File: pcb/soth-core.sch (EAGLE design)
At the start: 1 part, among them U1 ATXMEGA32D4-AU

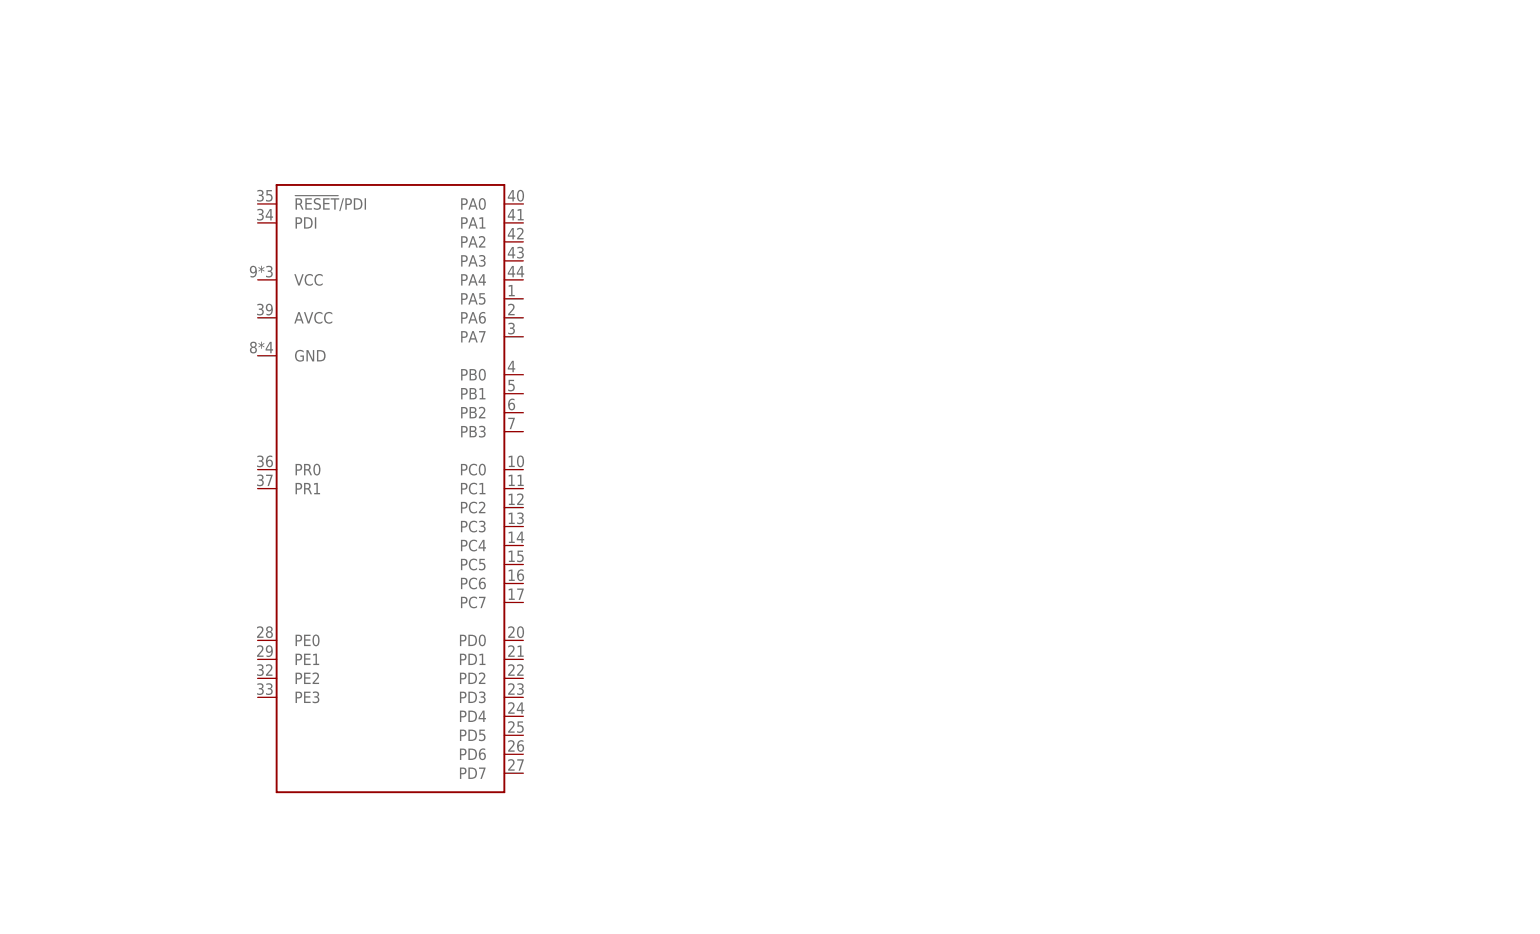
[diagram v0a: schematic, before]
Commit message: add current circuit schematic
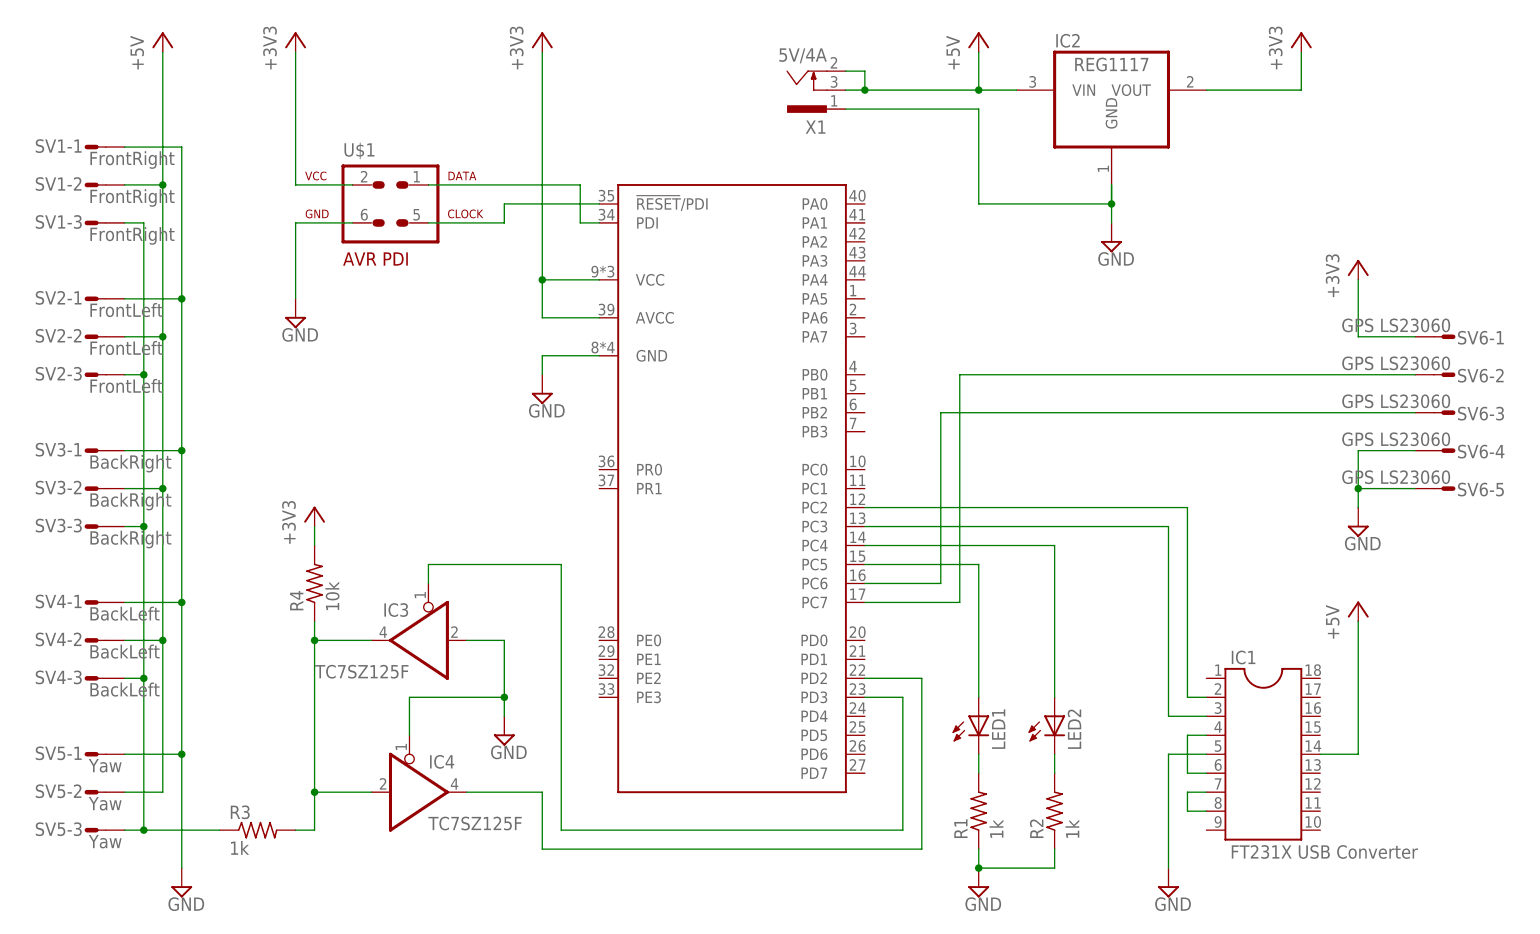
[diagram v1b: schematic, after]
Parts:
- added IC1: FT231X USB Converter, ic-package:DIL18S
- added IC2: REG1117, burr-brown:REG1117
- added IC3, IC4: TC7SZ125F, 74xx-little-de:74AHC1G125DBV
- added LED1, LED2: (no value), led:LED
- added R1, R2, R3: 1k, rcl:R-US_R0805
- added R4: 10k, rcl:R-US_R0805
- added SV1: FrontRight, con-amp-mt:S03P
- added SV2: FrontLeft, con-amp-mt:S03P
- added SV3: BackRight, con-amp-mt:S03P
- added SV4: BackLeft, con-amp-mt:S03P
- added SV5: Yaw, con-amp-mt:S03P
- added SV6: GPS LS23060, con-amp-mt:S05P
- added U$1: AVR-PDIVERT, atmega-atxmega:AVR-PDIVERT
- added X1: 5V/4A, con-conrad:733980-62
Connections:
- new net +3V3: IC2.VOUT, R4.2, SV6-1.S, U$1.2, U1.AVCC, U1.VCC
- new net +5V: IC1.14, IC2.VIN, SV1-2.S, SV2-2.S, SV3-2.S, SV4-2.S, SV5-2.S, X1.2, X1.3
- new net GND: IC1.5, IC2.GND, IC3A.I, IC4A.OE, R1.1, R2.1, SV1-1.S, SV2-1.S, SV3-1.S, SV4-1.S, SV5-1.S, SV6-4.S, SV6-5.S, U$1.6, U1.GND, X1.1
- new net N$1: R3.1, SV1-3.S, SV2-3.S, SV3-3.S, SV4-3.S, SV5-3.S
- new net N$10: IC1.2, U1.PC2
- new net N$11: IC1.3, U1.PC3
- new net N$12: IC1.7, IC1.8
- new net N$13: IC1.4, IC1.6
- new net N$14: SV6-3.S, U1.PC6
- new net N$15: IC3A.OE, U1.PD3
- new net N$17: IC3A.O, IC4A.I, R3.2, R4.1
- new net N$2: LED1.A, U1.PC5
- new net N$3: LED2.A, U1.PC4
- new net N$4: LED1.C, R1.2
- new net N$5: U$1.5, U1.!RESET!/PDI
- new net N$6: U$1.1, U1.PDI
- new net N$7: LED2.C, R2.2
- new net N$8: IC4A.O, U1.PD2
- new net N$9: SV6-2.S, U1.PC7
